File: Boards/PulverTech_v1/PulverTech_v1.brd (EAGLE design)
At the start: 95.9 x 61.6 mm, 40 parts, among them IC1 786TV, K1 G5LE, P1 FSMCD, Q1 16.0 mHz, Q4 BC548, Q6 IRF540, Q7 IRF540, Q8 IRF9530, Q9 IRF9530, U1 ATMEGA328P-PU

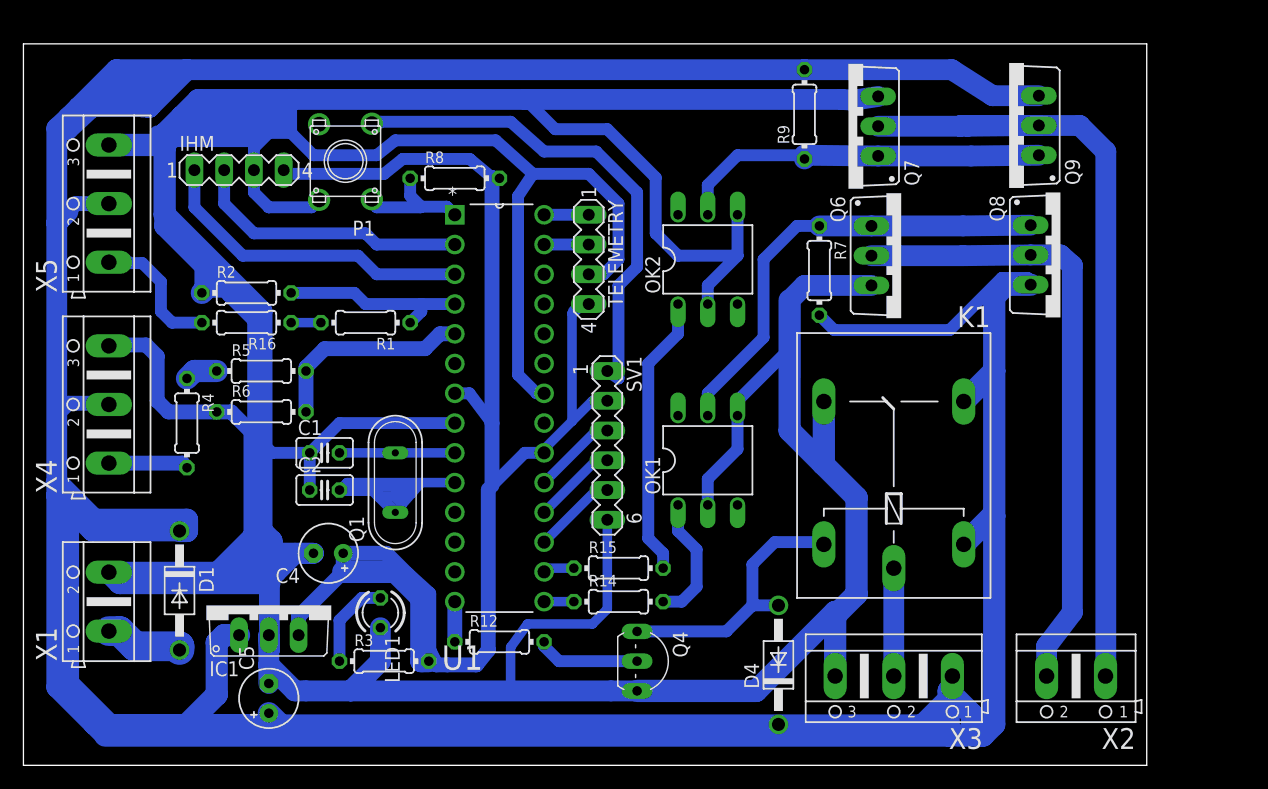
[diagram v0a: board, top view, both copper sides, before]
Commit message: final project updates
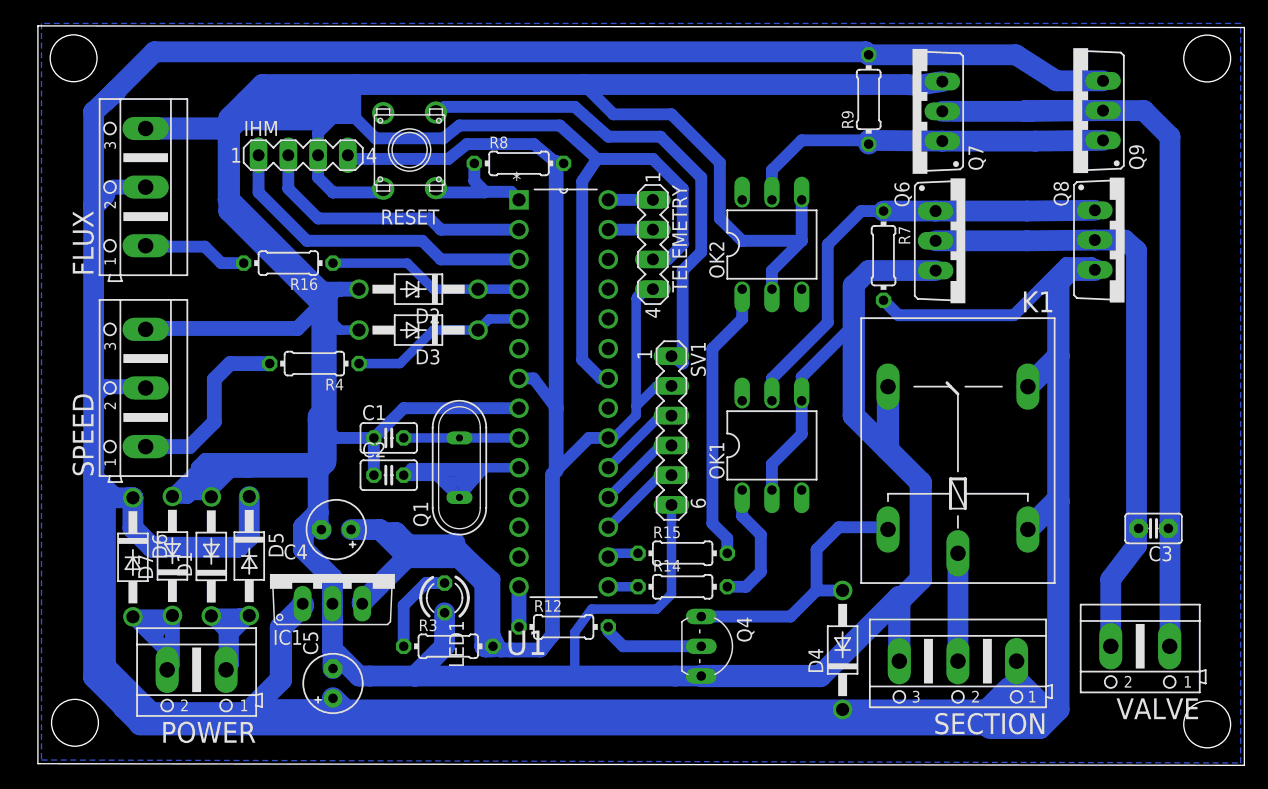
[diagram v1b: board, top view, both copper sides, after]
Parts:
- removed P1: FSMCD, switch-misc:FSMCD
- removed R1, R2, R5, R6: 10k, eagle-ltspice:0204/7
- removed X1, X2: (no value), con-ptr500:AK500/2
- removed X3, X4, X5: (no value), con-ptr500:AK500/3
- added C3: 100nF, capacitor-wima:C2.5-2
- added D2, D3: 1N4733, diode:DO41Z10
- added D5, D6, D7: 1N4007, diode:DO41-10
- added FLUX, SECTION, SPEED: (no value), con-ptr500:AK500/3
- added POWER, VALVE: (no value), con-ptr500:AK500/2
- added RESET: FSMCD, switch-misc:FSMCD
- R16, R4: value 10k -> 30k
- moved R4 12.0 mm to (23.3, 34.3), turned to 180 degrees
- moved R16 6.21 mm to (21.0, 42.9)
- moved IC1 6.06 mm to (24.8, 16.3)
- moved Q8 5.62 mm to (92.4, 44.8)
- moved Q9 5.62 mm to (88.0, 55.9)
- moved R7 5.62 mm to (71.8, 43.5)
- moved TELEMETRY 5.62 mm to (52.1, 44.5)
- moved K1 5.62 mm to (78.2, 27.6)
- moved LED1 5.62 mm to (34.4, 14.3)
- moved R14 5.62 mm to (54.7, 15.2)
- moved R15 5.62 mm to (54.7, 18.1)
- moved SV1 5.62 mm to (53.7, 28.6)
- moved U1 5.62 mm to (48.3, 15.2)
- moved Q6 5.62 mm to (78.8, 44.8)
- moved Q7 5.62 mm to (74.3, 55.8)
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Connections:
- removed net N$31: R4.1, R5.1
- net GND: now also D1.A, D2.A, D3.A, D7.A, FLUX.3, RESET.P$3, SECTION.3, SPEED.3; no longer P1.P$3, R2.1, R6.1, X1.2, X3.3, X4.3, X5.3
- net GND2: now also SECTION.2; no longer X3.2
- net MOTOR_A: now also C3.2, VALVE.2; no longer X2.2
- net MOTOR_B: now also C3.1, VALVE.1; no longer X2.1
- net N$12: now also FLUX.1; no longer X5.1
- net N$4: now also D1.C, D5.A, POWER.1; no longer R1.2, R16.1
- net N$5: now also D6.A, D7.C, POWER.2; no longer D1.A, X1.1
- net N$8: now also SPEED.1; no longer X4.1
- net RESET: now also RESET.P$1; no longer P1.P$1
- net RST_ICSP: now also RESET.P$2; no longer P1.P$2
- net SENSOR_FLUX: now also D2.C, R16.1; no longer R1.1, R2.2
- net SENSOR_IND: now also D3.C, R4.1; no longer R5.2, R6.2
- net VIN: now also D5.C, D6.C, FLUX.2, SECTION.1, SPEED.2; no longer D1.C, X3.1, X4.2, X5.2
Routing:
- net VIN: track 469.3 -> 452.6 mm
- net GND: track 564.7 -> 550.0 mm
- net N$4: track 2.54 -> 15.6 mm
- net N$5: track 6.89 -> 16.1 mm
- net N$8: track 6.83 -> 15.7 mm
- net VCC: track 133.1 -> 138.6 mm
- net N$31: track 2.80 -> 0.00 mm
- net N$12: track 13.1 -> 10.5 mm
- net SENSOR_IND: track 17.7 -> 15.2 mm
- added copper zone on layer 16, net GROUNDING
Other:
- board size 95.9 x 61.6 mm -> 103 x 63.1 mm
